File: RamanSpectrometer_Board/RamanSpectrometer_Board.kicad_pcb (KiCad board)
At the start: 2 copper layers, 49.3 x 90.9 mm, 33 parts, among them J1 RJ45_LED_Shielded, Q1 BSS138, Q2 BSS138, Q3 BSS138, Q4 BSS138, Q5 BSS138, U1 Teensy4.1_DEV-16771, U2 OKI 12V-5V, U3 OKI 5V-3V

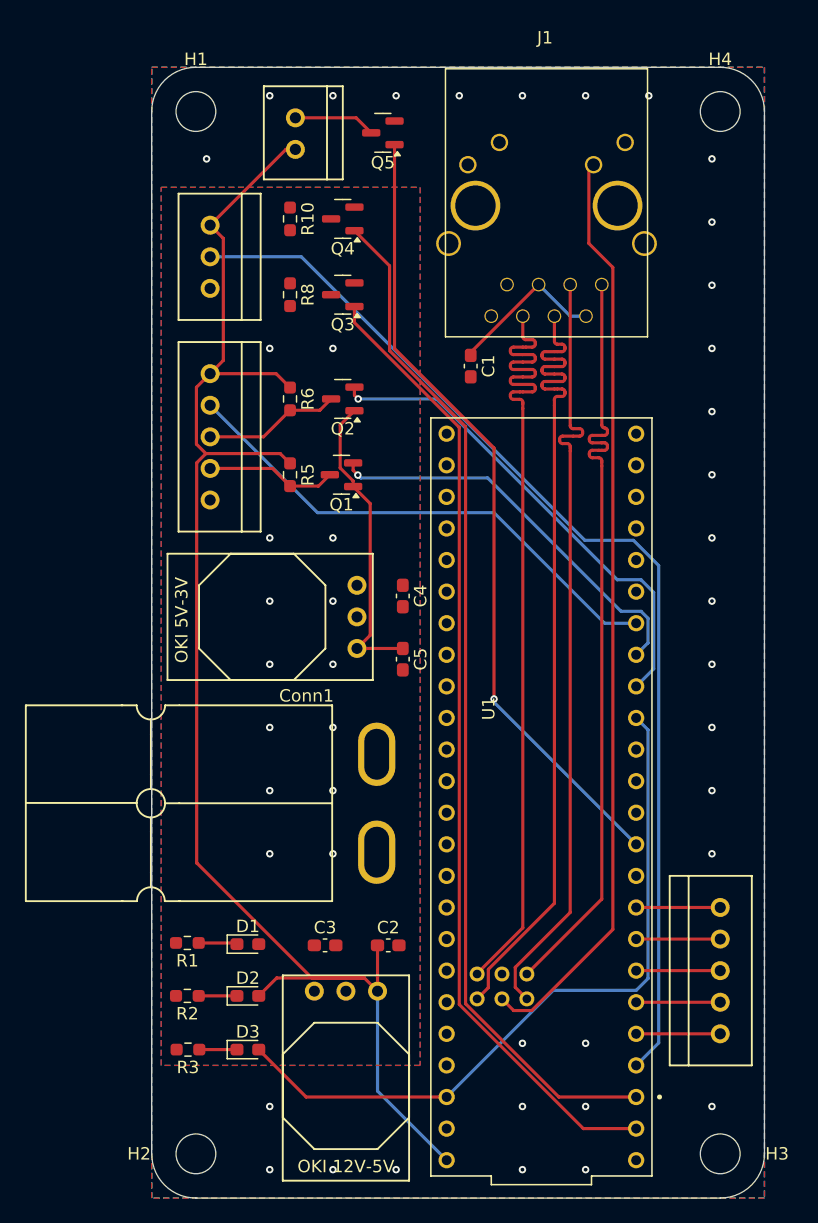
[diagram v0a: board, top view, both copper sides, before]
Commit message: PCB Raman again
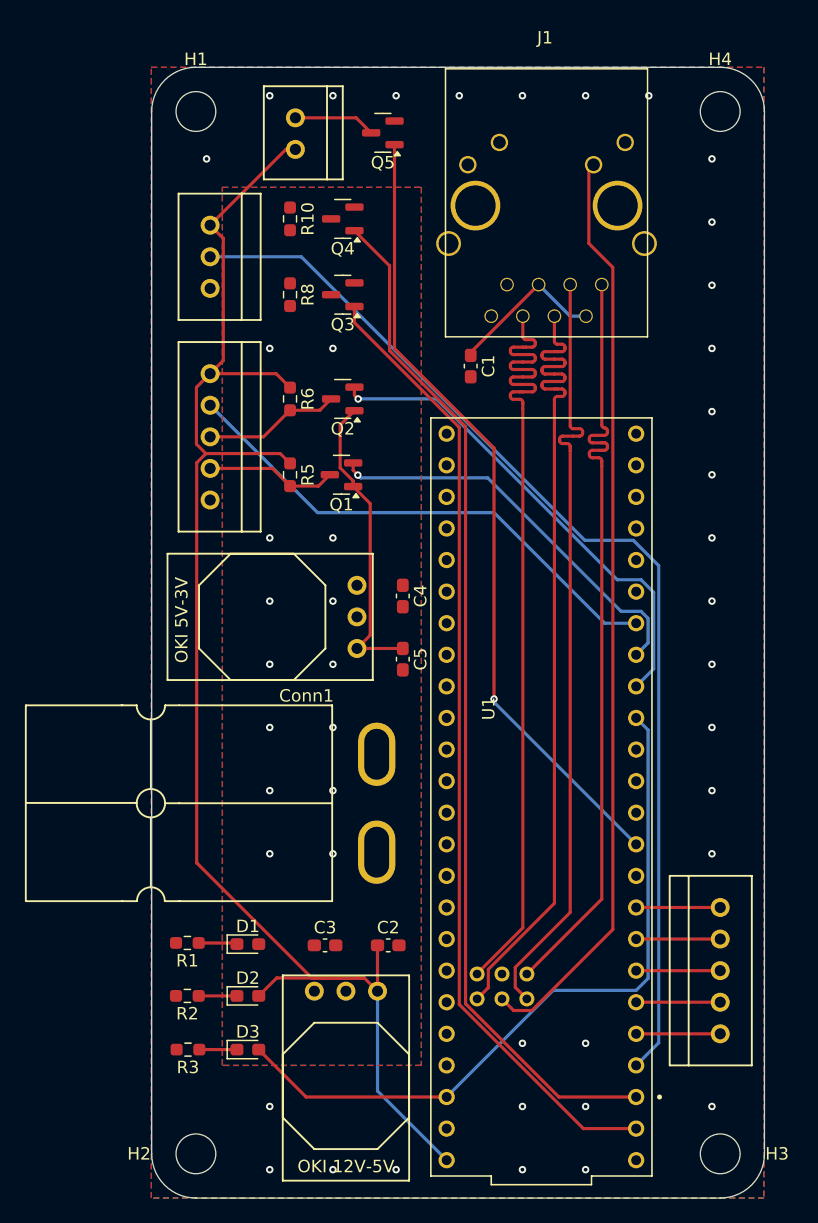
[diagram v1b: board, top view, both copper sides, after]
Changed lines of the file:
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@@
 		(net 4)
 		(net_name "+12V")
-		(layer "F.Cu")
+		(layers "F&B.Cu")
 		(hatch edge 0.5)
 		(priority 2)
-		(connect_pads
+		(connect_pads yes
 			(clearance 0.5)
 		)
 		(min_thickness 0.25)
 		(filled_areas_thickness no)
-		(fill yes
+		(fill
 			(thermal_gap 0.5)
 			(thermal_bridge_width 0.5)
@@
 		(polygon
 			(pts
-				(xy 143.667 53.084) (xy 164.495 53.084) (xy 164.495 123.696) (xy 143.667 123.696)
+				(xy 148.59 53.086) (xy 164.592 53.084) (xy 164.592 123.696) (xy 148.59 123.698)
 			)
 		)
@@
 		(polygon
 			(pts
-				(xy 142.905 43.432) (xy 192.181 43.432) (xy 192.181 134.364) (xy 142.905 134.364)
+				(xy 142.875 43.432) (xy 192.151 43.432) (xy 192.151 134.364) (xy 142.875 134.364)
 			)
 		)
-	)
-	(zone
-		(net 4)
-		(net_name "+12V")
-		(layer "B.Cu")
-		(hatch edge 0.5)
-		(priority 3)
-		(connect_pads
-			(clearance 0.5)
-		)
-		(min_thickness 0.25)
-		(filled_areas_thickness no)
-		(fill yes
-			(thermal_gap 0.5)
-			(thermal_bridge_width 0.5)
-		)
-		(polygon
-			(pts
-				(xy 143.667 53.084) (xy 164.495 53.084) (xy 164.495 123.696) (xy 143.667 123.696)
-			)
-		)
-	)
-	(zone
-		(net 2)
-		(net_name "GND")
-		(layer "B.Cu")
-		(hatch edge 0.5)
-		(priority 1)
-		(connect_pads
-			(clearance 0.5)
-		)
-		(min_thickness 0.25)
-		(filled_areas_thickness no)
-		(fill yes
-			(thermal_gap 0.5)
-			(thermal_bridge_width 0.5)
-		)
-		(polygon
-			(pts
-				(xy 142.905 43.432) (xy 192.181 43.432) (xy 192.181 134.364) (xy 142.905 134.364)
-			)
-		)
